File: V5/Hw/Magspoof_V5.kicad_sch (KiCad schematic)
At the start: 35 parts, among them J2 SWD, P1 USB_C_Plug_USB2.0, Q1 DMG3415U-7, SW1 ON, SW3 S1, SW4 SOURCE MAG, SW5 RESET, U1 CH552G, U2 AP2112K-3.3, U3 TC4424, U5 MCP73831

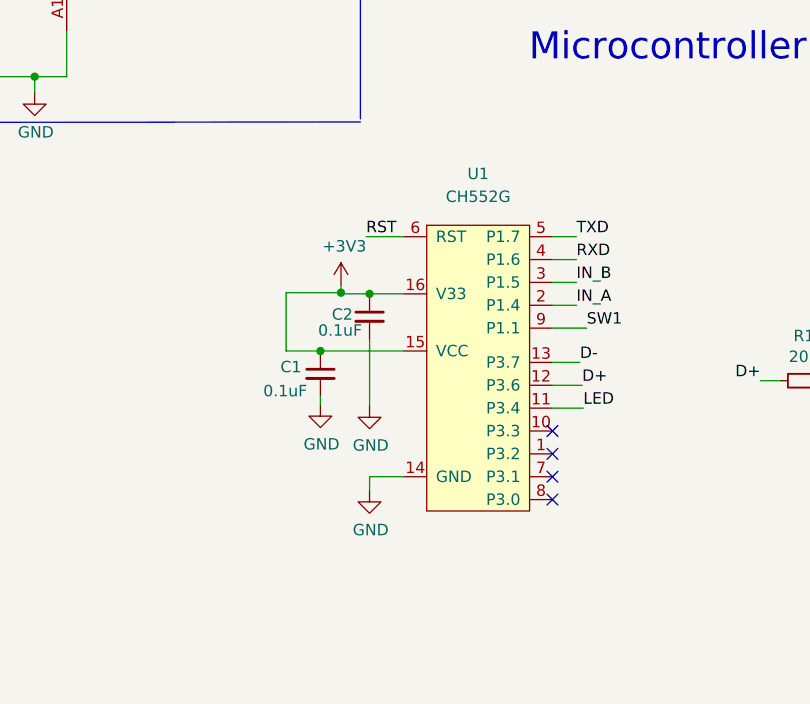
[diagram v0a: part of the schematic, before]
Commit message: feat(hw): TX and RX pins updated
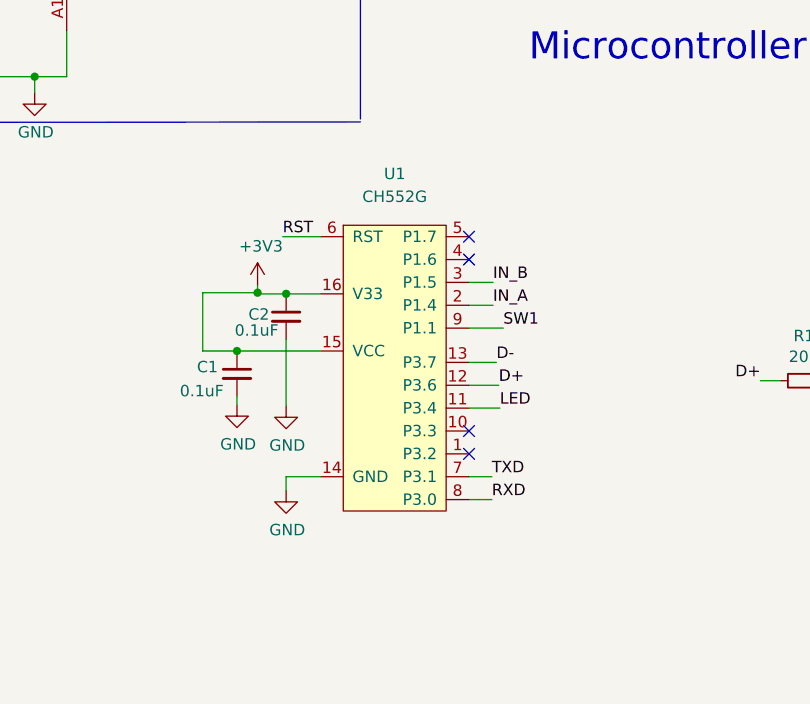
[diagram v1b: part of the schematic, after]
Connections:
- net RXD: now also U1.8 (P3.0); no longer U1.4 (P1.6)
- net TXD: now also U1.7 (P3.1); no longer U1.5 (P1.7)
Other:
- moved on the sheet: C1, C2, U1
